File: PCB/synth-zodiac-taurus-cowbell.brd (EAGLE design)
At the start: 76.1 x 72.4 mm, 63 parts, among them Q1 NPN, Q2 NPN, SW1 Push Switch, U1 TL071, U3 ATmega328P-AU, X1 16MHz, X2 16MHz

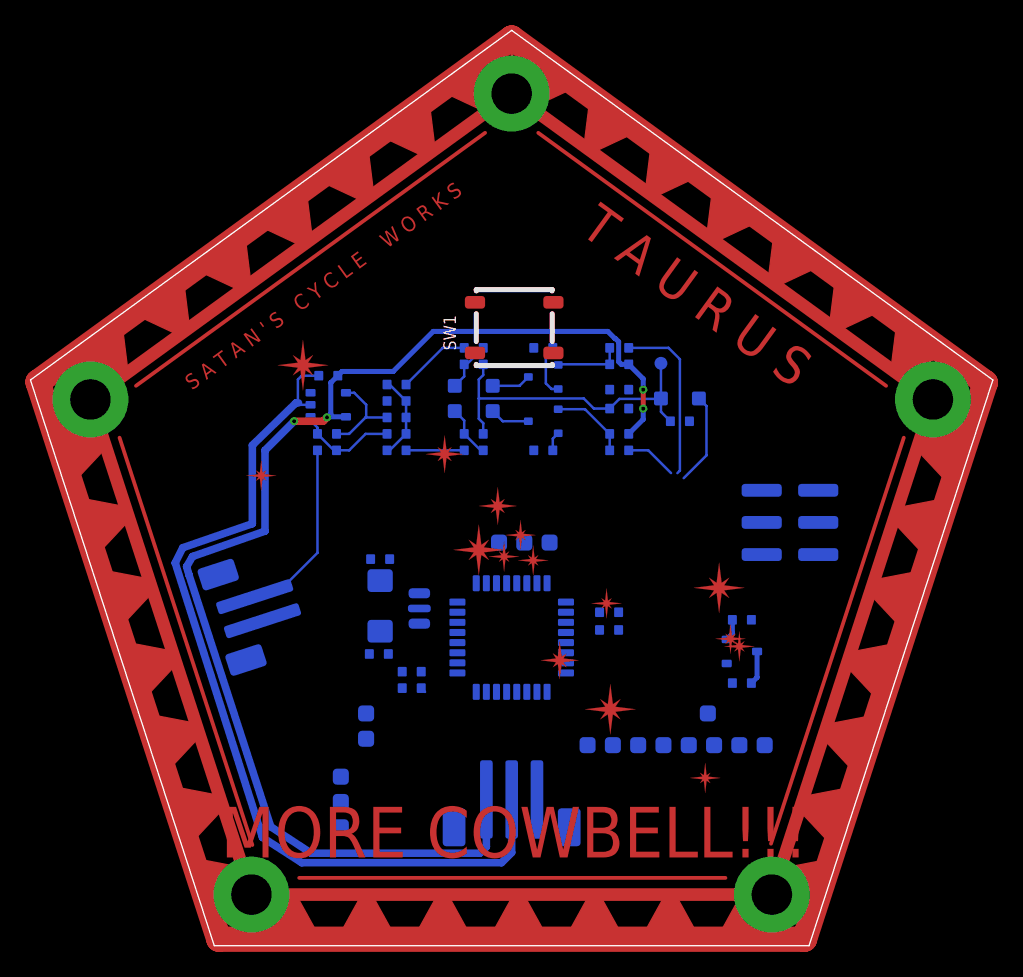
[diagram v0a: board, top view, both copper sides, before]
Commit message: Work in progress for rev A,  VCO rev.B
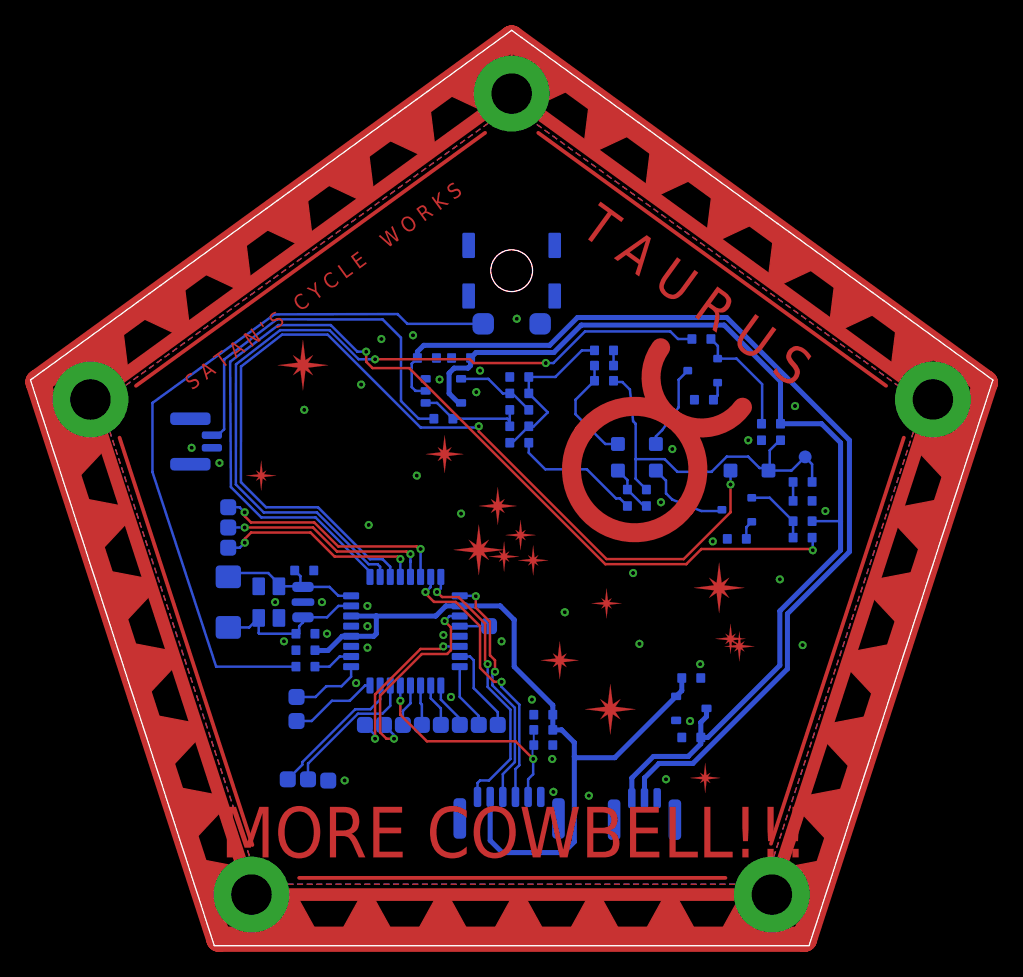
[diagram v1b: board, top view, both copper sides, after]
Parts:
- removed R16: 100, rlc:0603-RES
- removed SW1: Push Switch, switch-smd:B3SN
- added C16, C17: 0.1uF, rlc:0603-CAP
- added COW: SPST, TACT, MOM, switch-smd:B3FS-BACKMOUNT
- added GLYPH1: (no value), circuit-monkey-zodiac:TAURUS-GLYPH
- added R14: 100, rlc:0603-RES
- added X3: 16MHz, xtal:32X25
- COW2VCA: value 2-pin, VT, SMT -> JST, SH, 2P; device con-jst:B2B-PH-SM4 -> con-jst:BM02B-SRSS-TB
- ICSP: value (none) -> Connector, 6P, SM, VT; device con-headers:MA03X2-VT-SMD -> con-jst:BM06B-SRSS-TB
- PWR: value JST, 3P, VT, SMT -> JST SM 3P; device con-jst:B3B-PH-SM4 -> con-jst:BM03B-SRSS-TB
- moved ICSP 31.3 mm to (37.8, 12.1), turned to 180 degrees
- moved PB2 25.1 mm to (16.1, 35.3), turned to 0 degrees
- moved PB1 23.0 mm to (16.1, 33.7), turned to 0 degrees
- moved A0 21.2 mm to (36.9, 18.6)
- moved PB0 20.9 mm to (16.1, 32.1), turned to 0 degrees
- moved A1 20.7 mm to (35.4, 18.6)
- moved A2 20.2 mm to (33.9, 18.6)
- moved A3 19.7 mm to (32.4, 18.6)
- moved A4 19.2 mm to (30.9, 18.6)
- moved A5 18.7 mm to (29.4, 18.6)
- moved AREF 18.6 mm to (35.7, 25.9)
- moved A6 18.2 mm to (27.9, 18.6)
- moved A7 17.7 mm to (26.4, 18.6)
- moved C7 17.0 mm to (61.0, 35.8), turned to 180 degrees
- moved Q2 16.8 mm to (55.8, 35.1)
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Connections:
- net !RST: now also C17.1
- net -9V: now also C16.2; no longer C9.2
- net BTN_1: now also R14.1; no longer R16.1
- net GND: now also C16.1, C17.2, C9.2, COW.3; no longer SW1.3, SW1.4
- net N$11: now also COW.1, R14.2; no longer R16.2, SW1.1, SW1.2
- net XTAL1: now also X3.1
- net XTAL2: now also X3.3
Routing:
- net SQ_540: track 4.09 -> 81.0 mm, vias 0 -> 2
- net PULSE_1MS: track 7.29 -> 76.7 mm, vias 0 -> 2
- net +5V: track 1.74 -> 63.0 mm
- net N$11: track 0.00 -> 56.7 mm
- net SQ_800: track 13.5 -> 63.7 mm, vias 0 -> 2
- net MISO: track 0.00 -> 22.2 mm, vias 0 -> 2
- net MOSI: track 0.00 -> 22.1 mm, vias 0 -> 2
- net +9V: track 103.4 -> 83.1 mm, vias 4 -> 0
- net !RST: track 0.00 -> 19.8 mm, vias 0 -> 2
- net SCK: track 0.00 -> 19.0 mm, vias 0 -> 2
- net N$16: track 0.00 -> 19.0 mm, vias 0 -> 2
- net N$17: track 0.00 -> 17.1 mm, vias 0 -> 2
- net N$25: track 0.00 -> 16.6 mm, vias 0 -> 2
- net N$18: track 0.00 -> 16.6 mm, vias 0 -> 2
- net COW_OUT: track 14.5 -> 30.5 mm
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- added copper zone on layer 1, net GND
- added copper zone on layer 16, net GND
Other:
- board text added: "Rev. A"
- board text removed: "Rev. B"
